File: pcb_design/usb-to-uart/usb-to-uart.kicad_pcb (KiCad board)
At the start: 2 copper layers, 50 x 20 mm, 18 parts, among them IC2 L8050QLT1G, J1 Conn_01x06_Male, J2 TYPE-C-31-M-12, J3 Conn_01x04_Male, J4 Conn_01x04_Male, SW1 SW_MEC_5G

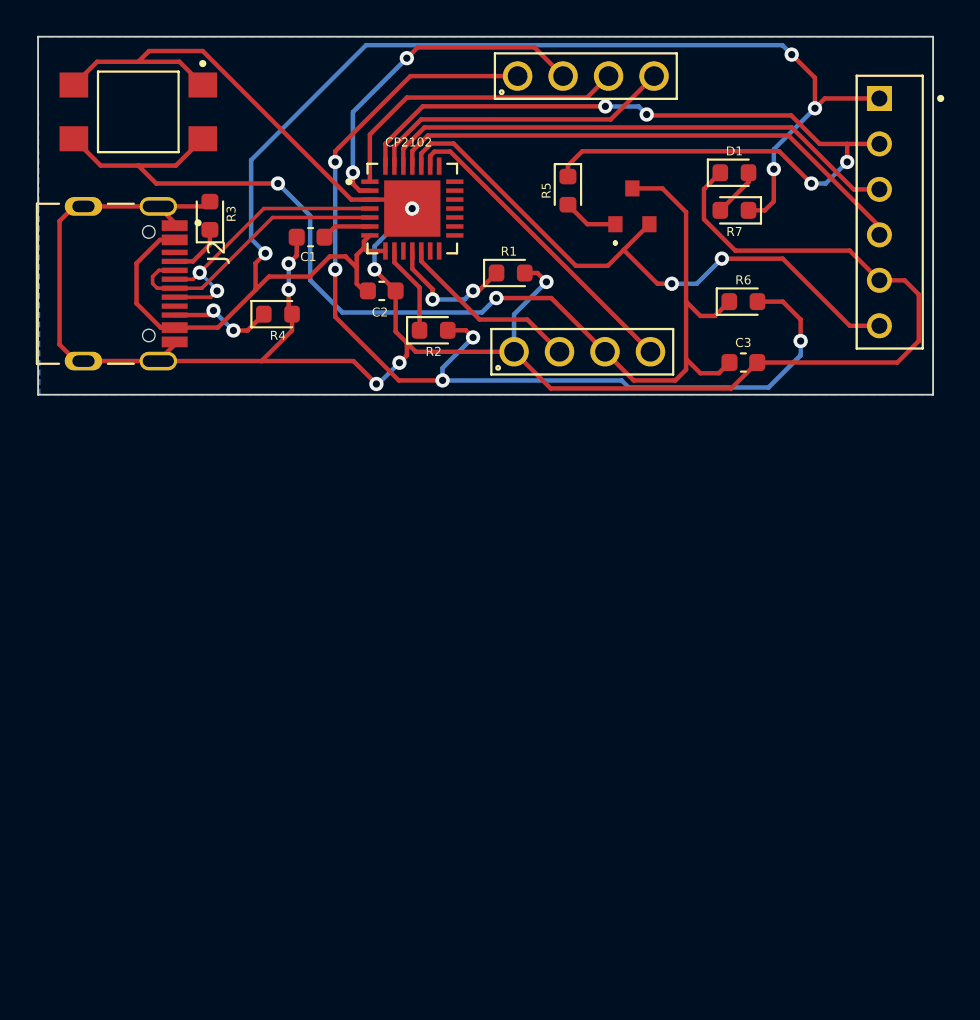
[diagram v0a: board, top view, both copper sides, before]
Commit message: PCB Completed
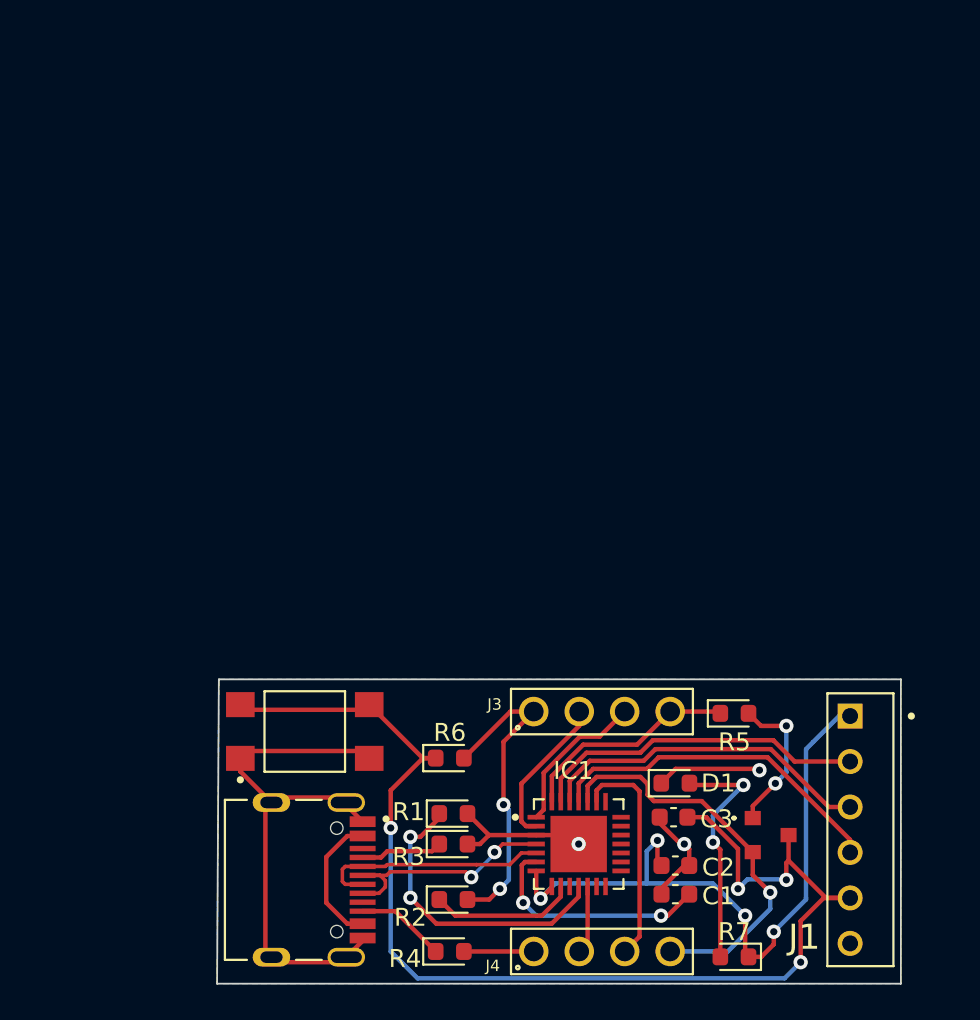
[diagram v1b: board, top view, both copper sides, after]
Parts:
- removed CP2102: CP2102, CP2102:QFN50P500X500X100-29N
- added IC1: CP2102, CP2102:QFN50P500X500X100-29N, F.Cu at (137.0, 109.3)
- moved C1 42.0 mm to (142.4, 112.1)
- moved R7 41.7 mm to (145.7, 115.6)
- moved R3 37.6 mm to (130.0, 109.3), turned to 0 degrees
- moved R4 36.9 mm to (129.8, 115.3)
- moved C2 36.0 mm to (142.4, 110.5)
- moved IC2 36.0 mm to (147.7, 108.8), turned to -90 degrees
- moved SW1 35.8 mm to (121.7, 103.0), turned to 90 degrees
- moved J3 35.5 mm to (138.3, 101.9)
- moved J2 34.9 mm to (119.8, 111.3)
- moved J1 34.5 mm to (152.2, 108.5)
- moved D1 34.3 mm to (142.4, 105.9)
- moved J4 33.5 mm to (138.3, 115.3)
- moved R2 31.8 mm to (130.0, 112.4)
- moved R5 30.6 mm to (145.7, 102.0), turned to 0 degrees
- moved R1 30.4 mm to (130.0, 107.6)
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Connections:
- J1 pad 2: DTR -> DSR
- J1 pad 5: GND -> EN
- J1 pad 6: RTS -> GND
- J3 pad 4: DSR -> DTR
- J4 pad 3: EN -> CTS
- J4 pad 4: CTS -> RTS
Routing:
- net GND: track 140.2 -> 55.4 mm, vias 7 -> 3
- net 3V3: track 59.1 -> 18.0 mm, vias 5 -> 2
- net DTR: track 49.4 -> 12.4 mm, vias 4 -> 0
- net 5V: track 80.9 -> 45.8 mm
- net RTS: track 34.7 -> 22.6 mm, vias 2 -> 1
- net Net-(D1-Pad2): track 2.75 -> 13.5 mm, vias 0 -> 2
- net TXD: track 29.5 -> 18.9 mm
- net RI: track 19.0 -> 8.42 mm, vias 2 -> 0
- net RXD: track 29.9 -> 19.4 mm
- net Net-(C1-Pad2): track 2.78 -> 13.1 mm, vias 0 -> 2
- net Net-(IC1-Pad11): track 7.36 -> 16.9 mm
- net DCD: track 17.3 -> 8.59 mm
- net SUSPEND: track 10.4 -> 3.82 mm
- net Net-(IC2-Pad1): track 3.10 -> 8.33 mm, vias 0 -> 2
- net CTS: track 17.6 -> 12.6 mm
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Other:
- board size 50 x 20 mm -> 38.2 x 17 mm
